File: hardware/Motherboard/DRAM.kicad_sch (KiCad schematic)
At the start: 26 parts, among them U11 74LS245, U12 74LS541, U13 74LS541, U14 74LS541, U15 74LS393, U16 MK4164N, U17 MK4164N, U18 MK4164N, U19 MK4164N, U2 74LS123, U20 MK4164N, U21 MK4164N, U22 MK4164N, U23 MK4164N, U24 74LS123, U25 74LS74, U26 74LS74, U28 74LS04, U29 74LS02, U71 74LS393, U8 74LS00

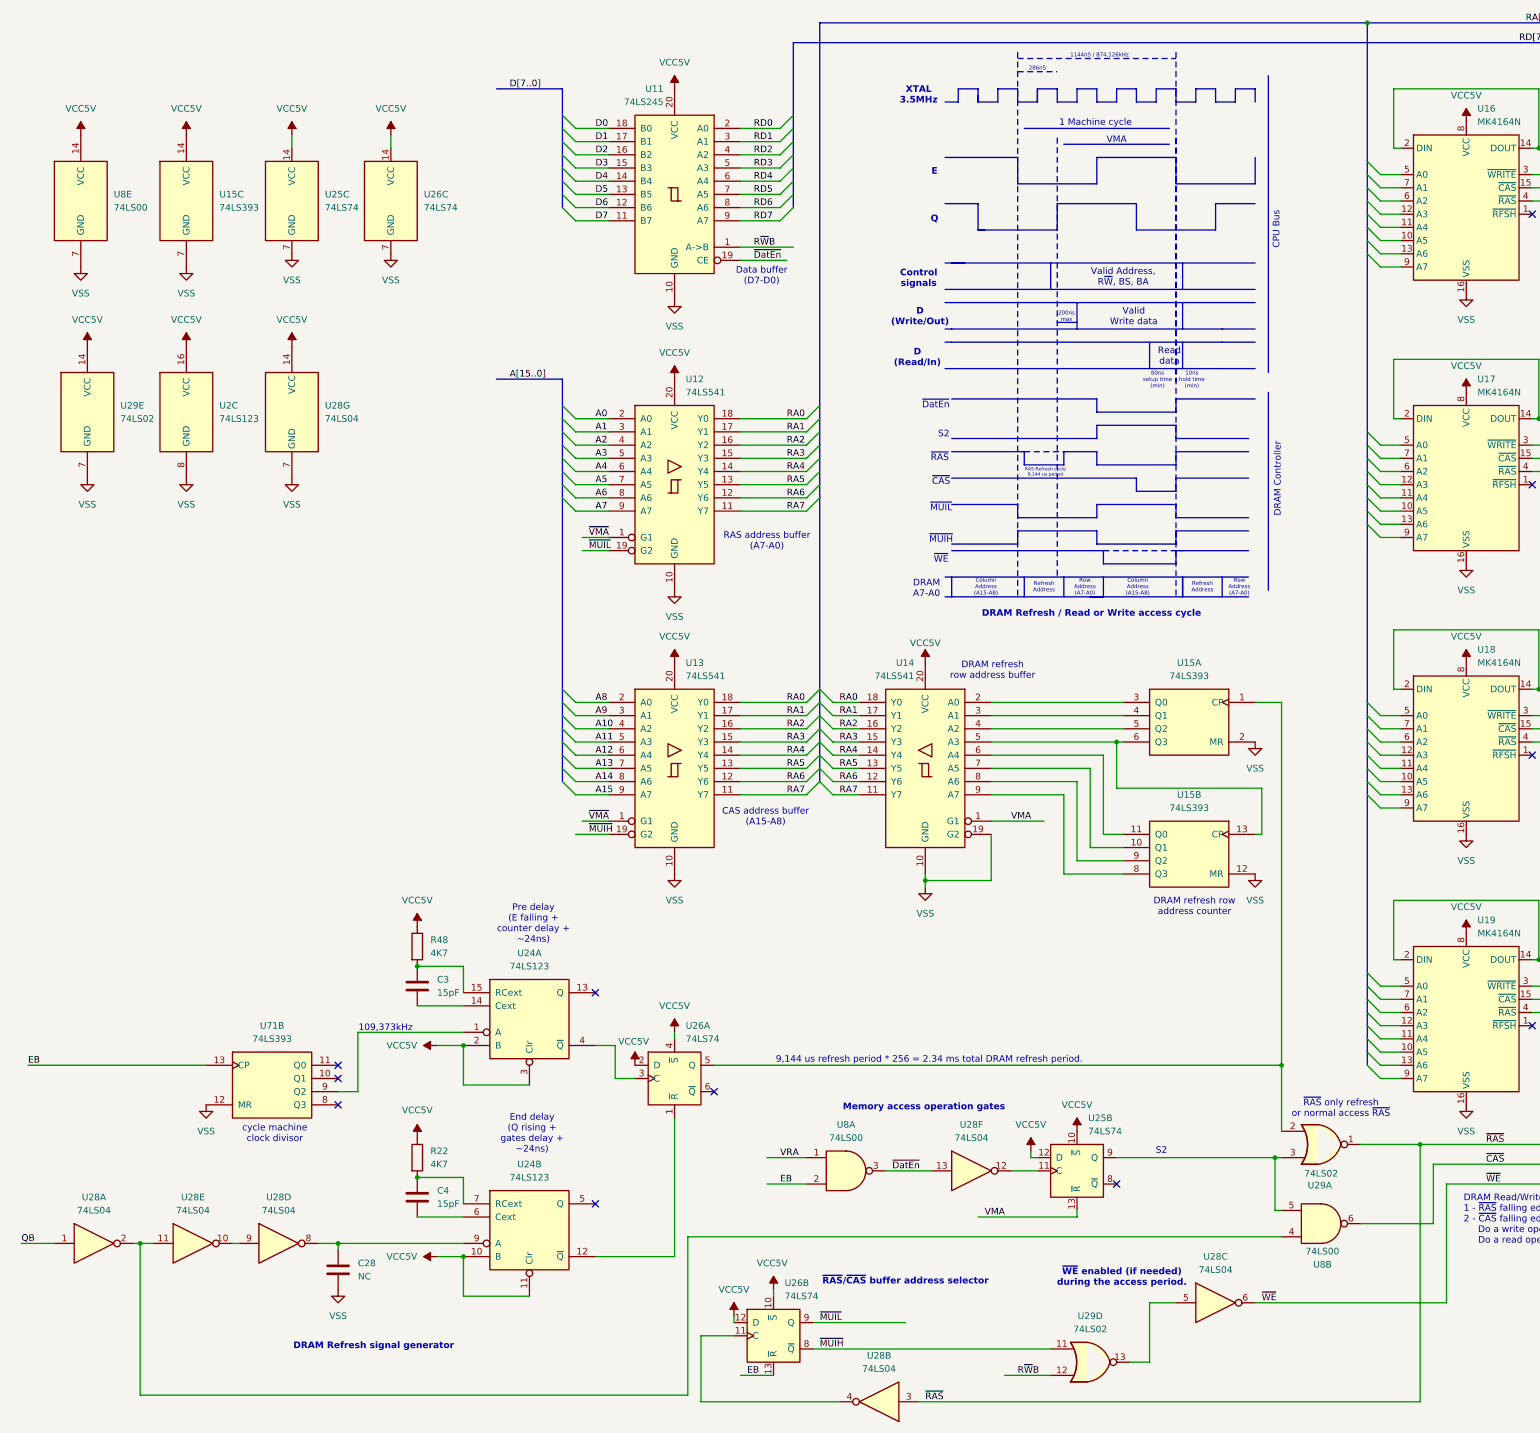
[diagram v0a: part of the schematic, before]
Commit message: WIP -rom pack
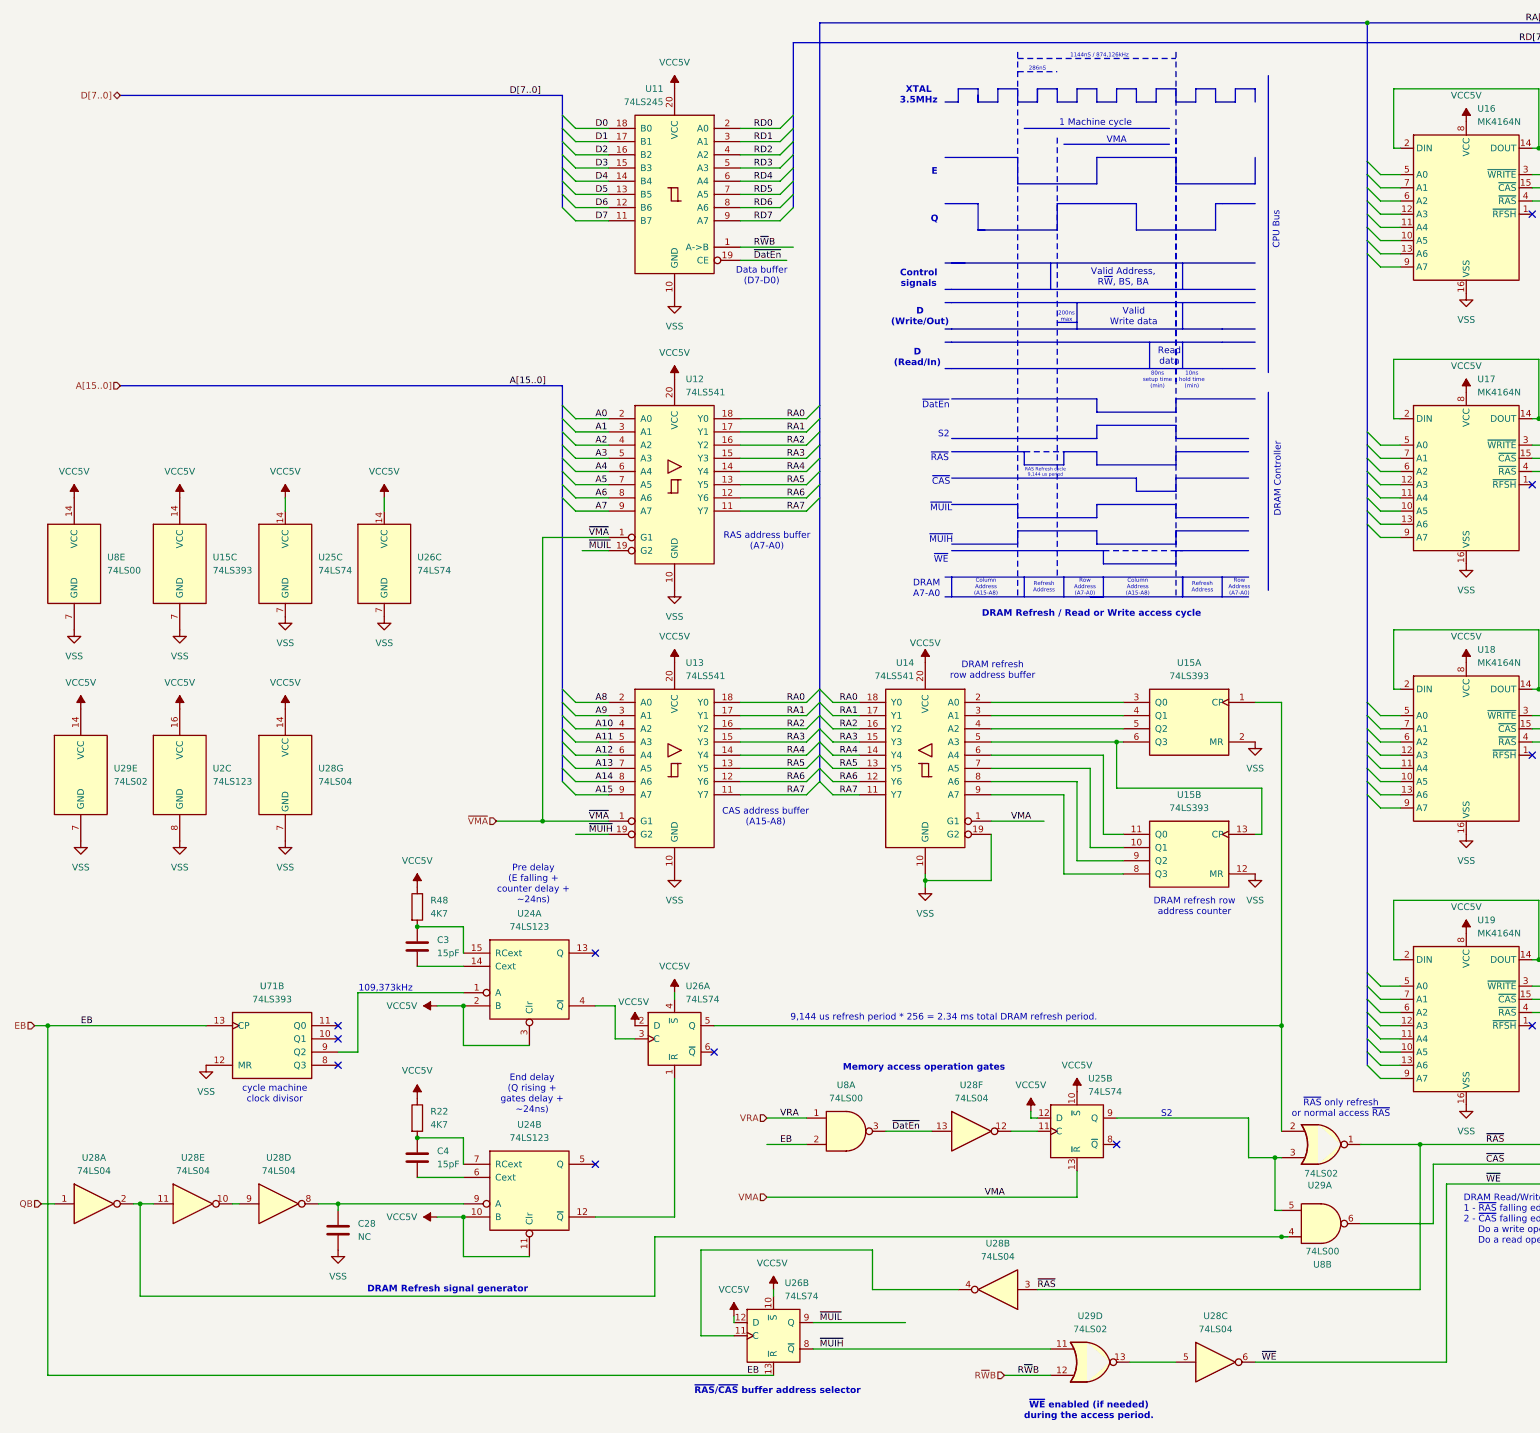
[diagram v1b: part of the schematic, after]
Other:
- moved on the sheet: C28, C3, C4, R22, R48, U15C, U24A, U24B, U25B, U25C, U26A, U26C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
